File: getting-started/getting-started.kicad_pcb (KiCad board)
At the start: 2 copper layers, 38.1 x 38.1 mm, 3 parts

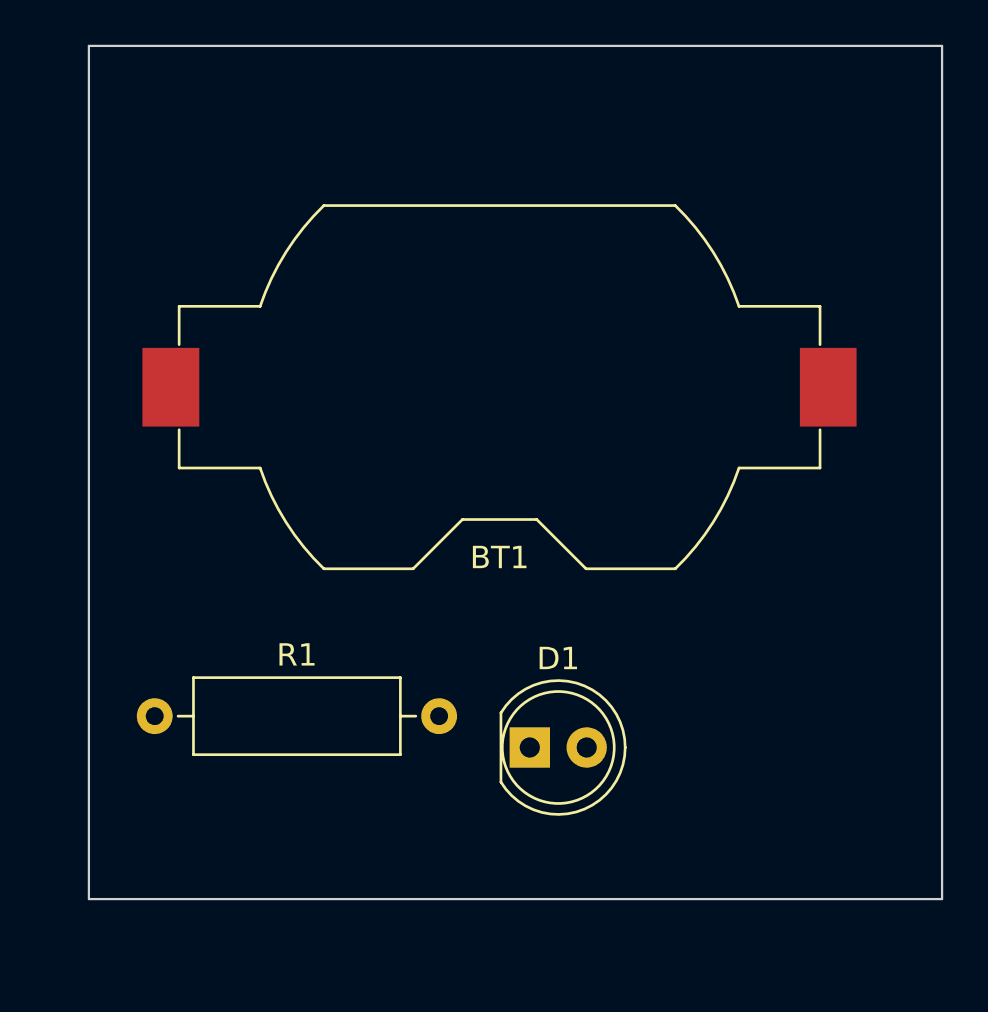
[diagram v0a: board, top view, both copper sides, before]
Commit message: Routing tracks
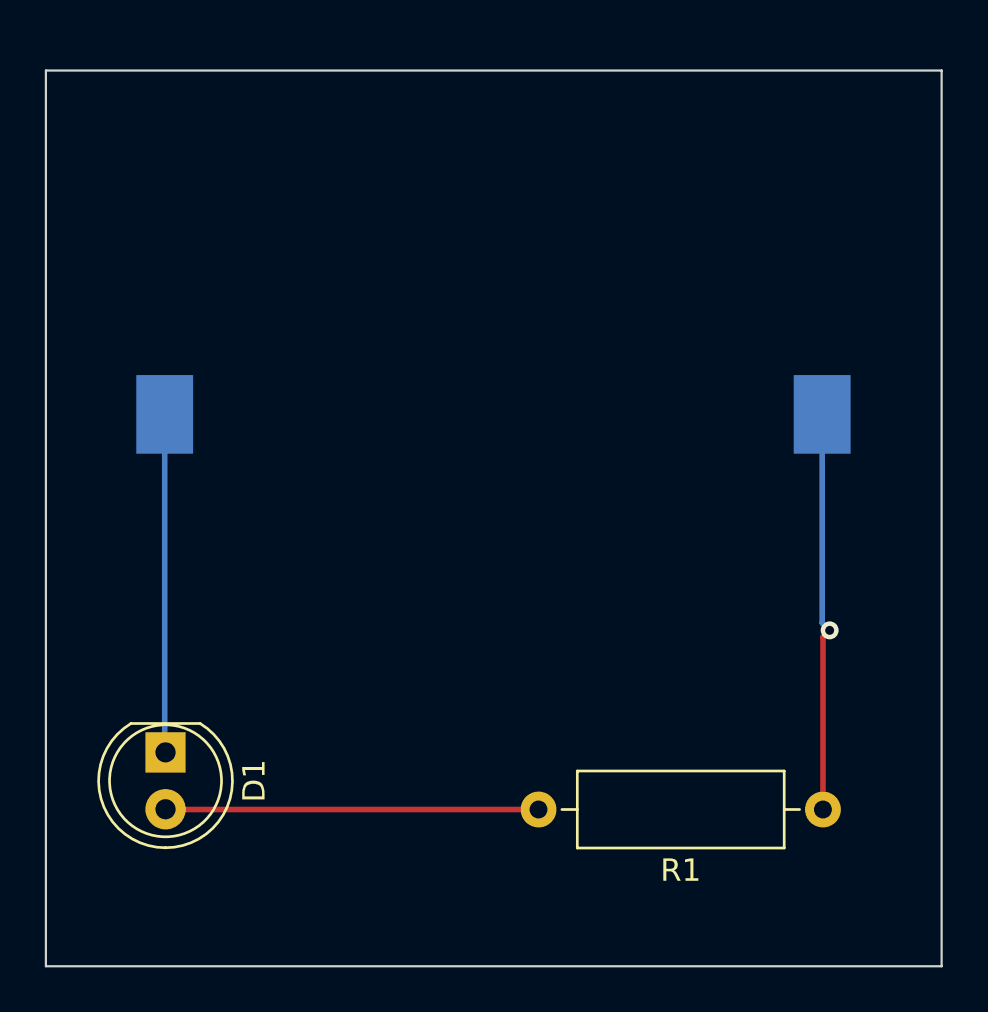
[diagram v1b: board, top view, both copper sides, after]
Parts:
- BT1: moved to B.Cu
- moved R1 30.1 mm to (154.7, 123.0), turned to 180 degrees
- moved D1 16.3 mm to (125.3, 120.4), turned to -90 degrees
- moved BT1 1.25 mm to (140.0, 105.4), turned to 180 degrees
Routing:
- net VCC: track 0.00 -> 17.9 mm, vias 0 -> 1
- net /led: track 0.00 -> 16.7 mm
- net GND: track 0.00 -> 15.1 mm
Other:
- board size 38.1 x 38.1 mm -> 40 x 40 mm
